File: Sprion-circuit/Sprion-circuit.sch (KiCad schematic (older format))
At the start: 0 parts

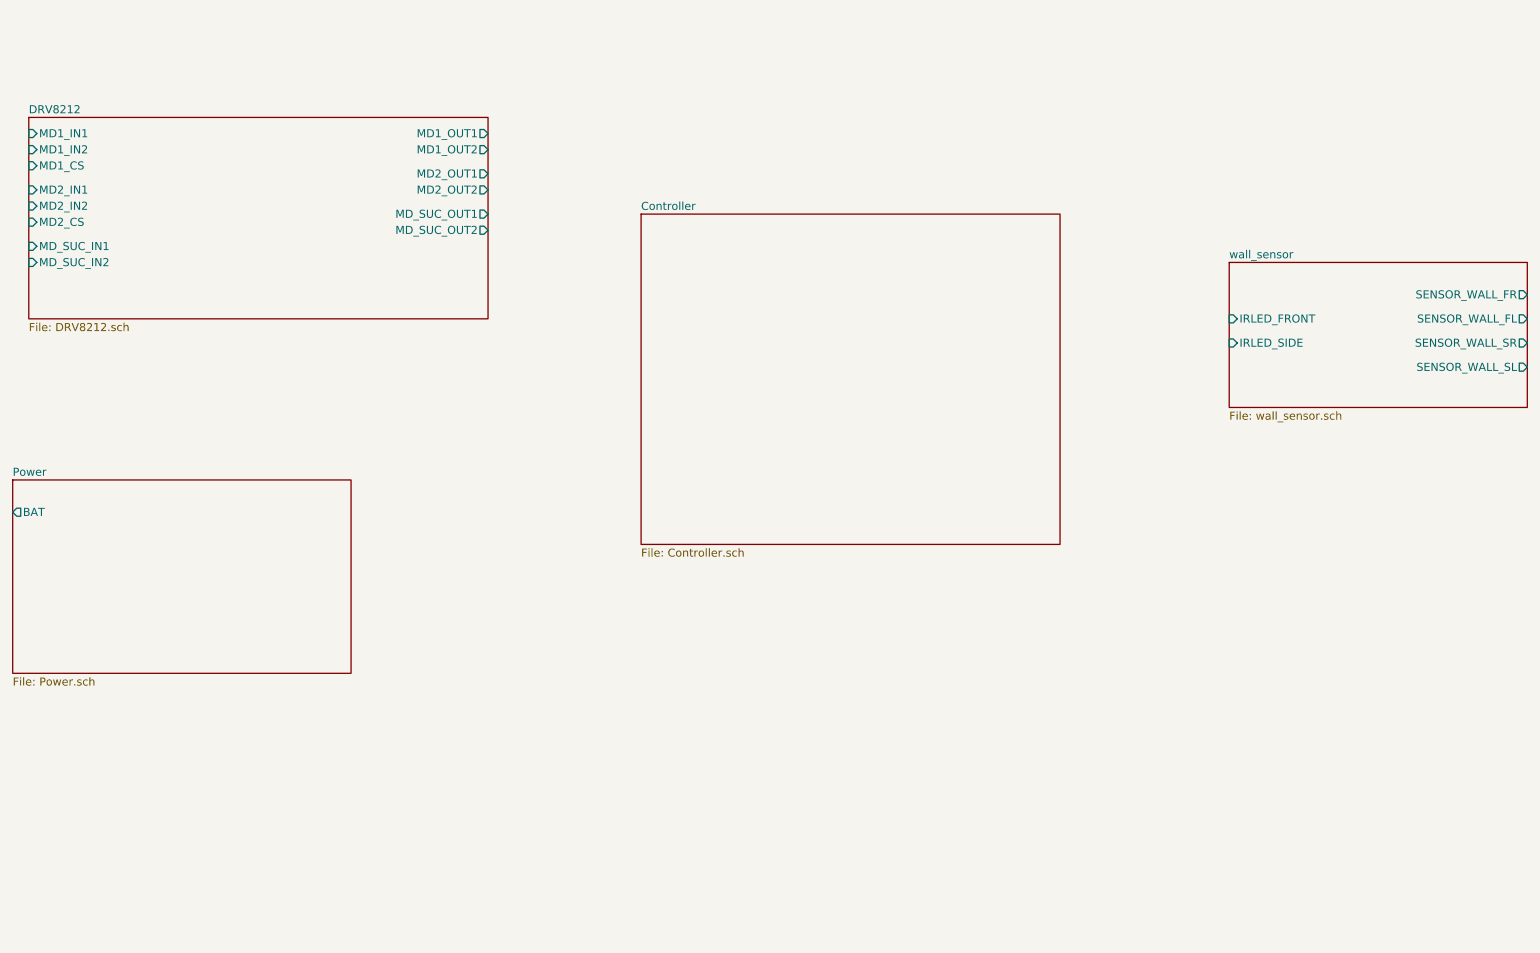
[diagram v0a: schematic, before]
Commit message: :fix　いろいろ
後で書きます
とりあえず寝ます
許してください
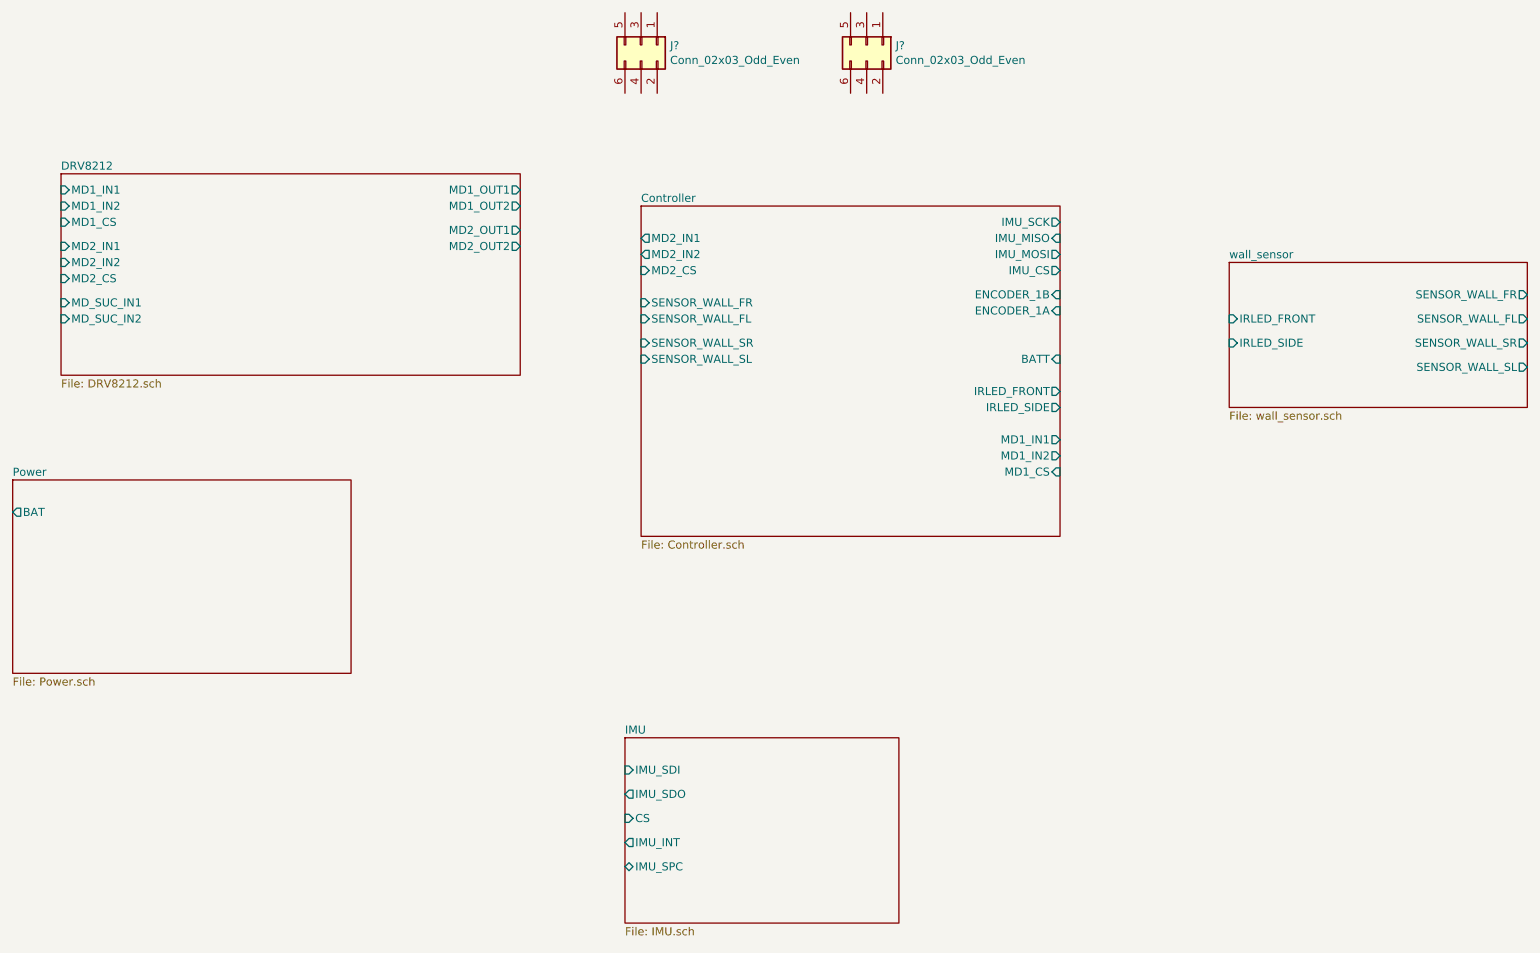
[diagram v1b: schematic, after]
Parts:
- added J? (x2): Conn_02x03_Odd_Even, symbol Connector_Generic:Conn_02x03_Odd_Even
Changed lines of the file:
@@
 $Descr A4 11693 8268
 encoding utf-8
-Sheet 1 5
+Sheet 1 6
 Title ""
 Date ""
@@
 Comment4 ""
 $EndDescr
-$Sheet
-S 1400 1500 2850 1250
-U 60E26C28
-F0 "DRV8212" 50
-F1 "DRV8212.sch" 50
-F2 "MD1_IN1" I L 1400 1600 50
-F3 "MD1_IN2" I L 1400 1700 50
-F4 "MD1_OUT1" O R 4250 1600 50
-F5 "MD1_OUT2" O R 4250 1700 50
-F6 "MD1_CS" I L 1400 1800 50
-F7 "MD2_IN1" I L 1400 1950 50
-F8 "MD2_IN2" I L 1400 2050 50
-F9 "MD2_OUT1" O R 4250 1850 50
-F10 "MD2_OUT2" O R 4250 1950 50
-F11 "MD_SUC_IN1" I L 1400 2300 50
-F12 "MD_SUC_IN2" I L 1400 2400 50
-F13 "MD_SUC_OUT1" O R 4250 2100 50
-F14 "MD_SUC_OUT2" O R 4250 2200 50
-F15 "MD2_CS" I L 1400 2150 50
-$EndSheet
 $Sheet
 S 1300 3750 2100 1200
@@
 F7 "SENSOR_WALL_SL" O R 10700 3050 50
 $EndSheet
+$Comp
+L Connector_Generic:Conn_02x03_Odd_Even J?
+U 1 1 61A7CC1C
+P 5200 1050
+F 0 "J?" V 5204 1230 50  0000 L CNN
+F 1 "Conn_02x03_Odd_Even" V 5295 1230 50  0000 L CNN
+F 2 "" H 5200 1050 50  0001 C CNN
+F 3 "~" H 5200 1050 50  0001 C CNN
+	1    5200 1050
+	0    1    1    0
+$EndComp
+$Comp
+L Connector_Generic:Conn_02x03_Odd_Even J?
+U 1 1 61A7F0D6
+P 6600 1050
+F 0 "J?" V 6604 1230 50  0000 L CNN
+F 1 "Conn_02x03_Odd_Even" V 6695 1230 50  0000 L CNN
+F 2 "" H 6600 1050 50  0001 C CNN
+F 3 "~" H 6600 1050 50  0001 C CNN
+	1    6600 1050
+	0    1    1    0
+$EndComp
 $Sheet
-S 5200 2100 2600 2050
+S 1600 1850 2850 1250
+U 60E26C28
+F0 "DRV8212" 50
+F1 "DRV8212.sch" 50
+F2 "MD1_IN1" I L 1600 1950 50
+F3 "MD1_IN2" I L 1600 2050 50
+F4 "MD1_OUT1" O R 4450 1950 50
+F5 "MD1_OUT2" O R 4450 2050 50
+F6 "MD1_CS" I L 1600 2150 50
+F7 "MD2_IN1" I L 1600 2300 50
+F8 "MD2_IN2" I L 1600 2400 50
+F9 "MD2_OUT1" O R 4450 2200 50
+F10 "MD2_OUT2" O R 4450 2300 50
+F11 "MD_SUC_IN1" I L 1600 2650 50
+F12 "MD_SUC_IN2" I L 1600 2750 50
+F15 "MD2_CS" I L 1600 2500 50
+$EndSheet
+$Sheet
+S 5200 2050 2600 2050
 U 60F363D5
 F0 "Controller" 50
 F1 "Controller.sch" 50
+F2 "IMU_SCK" O R 7800 2150 50
+F3 "IMU_MISO" I R 7800 2250 50
+F4 "IMU_MOSI" O R 7800 2350 50
+F5 "ENCODER_1B" I R 7800 2600 50
+F6 "ENCODER_1A" I R 7800 2700 50
+F7 "IMU_CS" O R 7800 2450 50
+F8 "BATT" I R 7800 3000 50
+F9 "IRLED_FRONT" O R 7800 3200 50
+F10 "IRLED_SIDE" O R 7800 3300 50
+F11 "MD1_IN1" O R 7800 3500 50
+F12 "MD1_IN2" O R 7800 3600 50
+F13 "MD2_IN1" O L 5200 2250 50
+F14 "MD2_IN2" O L 5200 2350 50
+F15 "MD1_CS" I R 7800 3700 50
+F16 "MD2_CS" I L 5200 2450 50
+F17 "SENSOR_WALL_FR" I L 5200 2650 50
+F18 "SENSOR_WALL_FL" I L 5200 2750 50
+F19 "SENSOR_WALL_SR" I L 5200 2900 50
+F20 "SENSOR_WALL_SL" I L 5200 3000 50
+$EndSheet
+$Sheet
+S 5100 5350 1700 1150
+U 61A9F6C1
+F0 "IMU" 50
+F1 "IMU.sch" 50
+F2 "IMU_SDI" I L 5100 5550 50
+F3 "IMU_SDO" O L 5100 5700 50
+F4 "CS" I L 5100 5850 50
+F5 "IMU_INT" O L 5100 6000 50
+F6 "IMU_SPC" B L 5100 6150 50
 $EndSheet
 $EndSCHEMATC
